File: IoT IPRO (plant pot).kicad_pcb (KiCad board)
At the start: 2 copper layers, 16 parts, among them J1 Barrel_Jack, Q1 Q_DUAL_NMOS_S1G1S2G2D1D1D2D2, U1 DS18S20, U3 AP9101C-SOT25

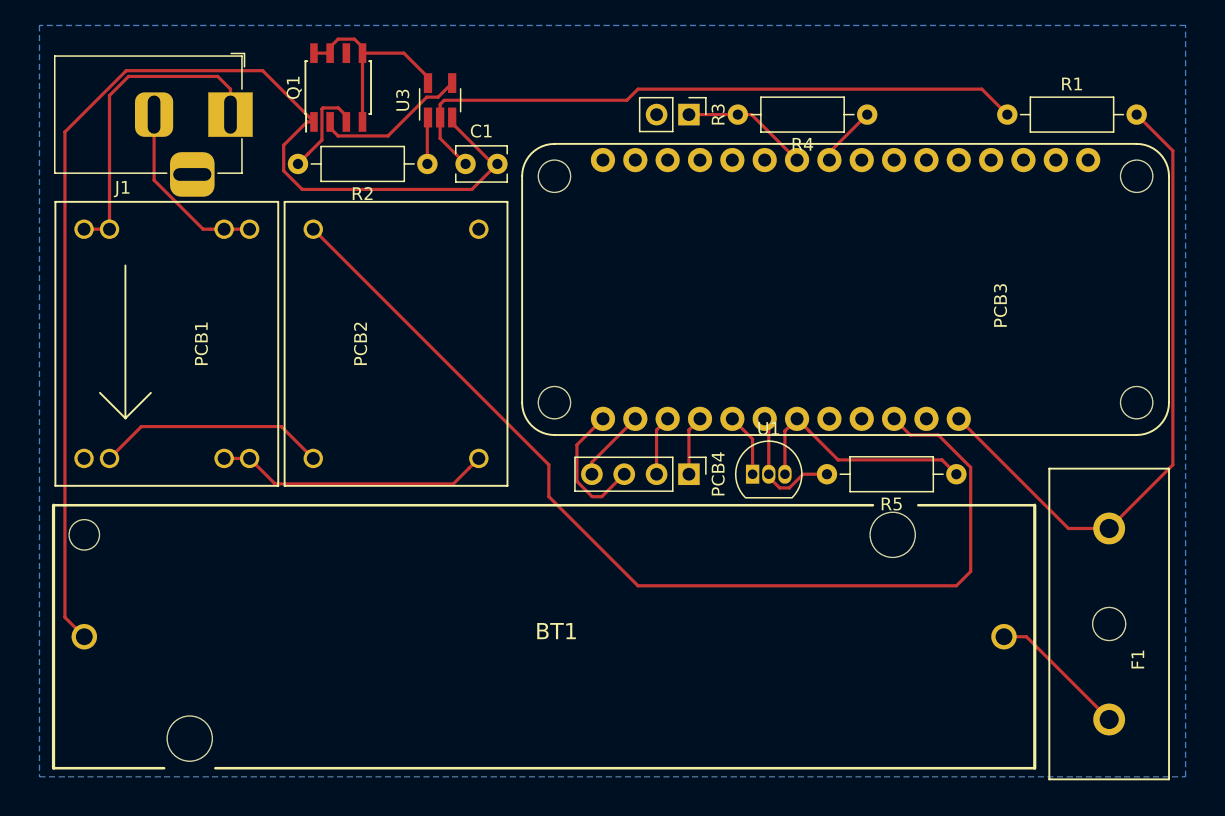
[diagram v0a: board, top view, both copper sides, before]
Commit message: Update PCB, PDFs
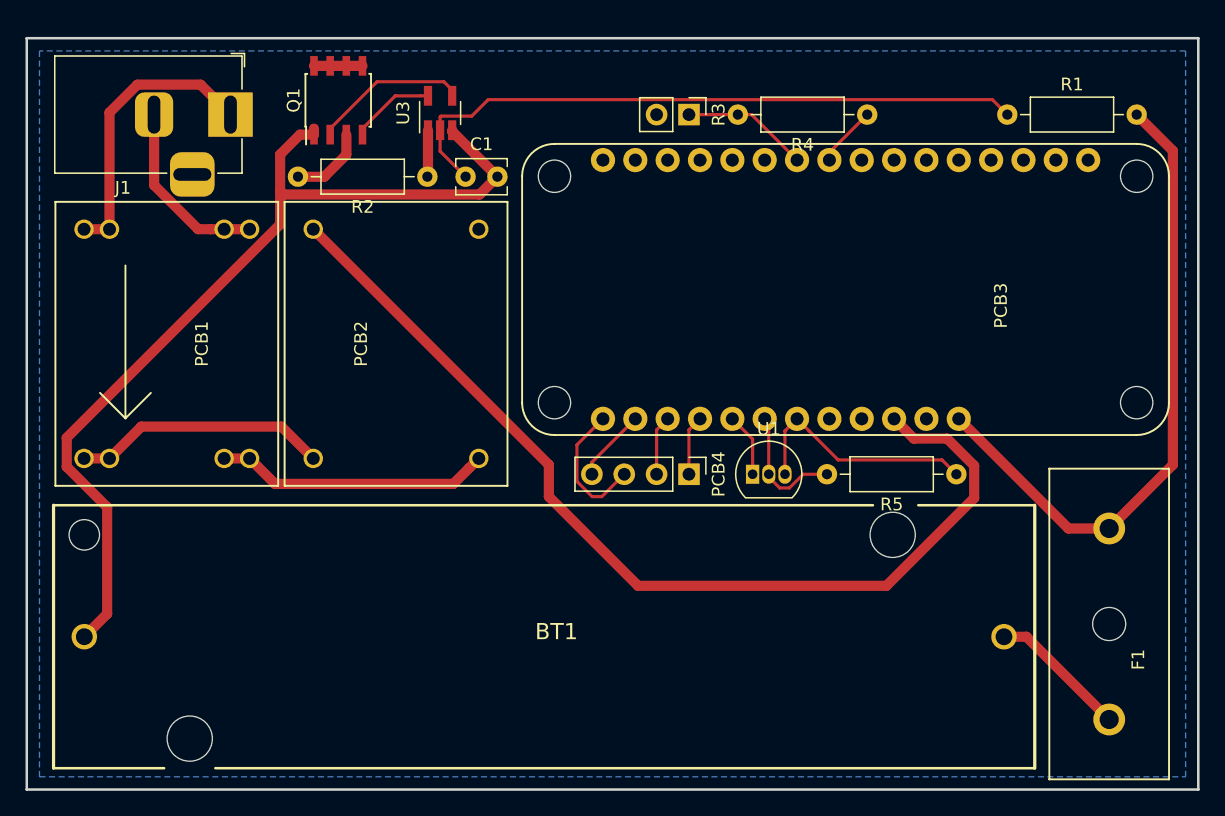
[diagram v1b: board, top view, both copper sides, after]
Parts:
- moved C1 1.00 mm to (92.5, 39.9)
- moved Q1 1.00 mm to (82.5, 33.9)
- moved R2 1.00 mm to (89.5, 39.9)
- moved U3 1.00 mm to (90.5, 34.9)
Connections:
- Q1 pad 5: Net-(Q1-Pad4) -> Net-(Q1-Pad5)
- Q1 pad 6: (no net) -> Net-(Q1-Pad5)
- Q1 pad 7: Net-(Q1-Pad4) -> Net-(Q1-Pad5)
- Q1 pad 8: Net-(Q1-Pad4) -> Net-(Q1-Pad5)
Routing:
- net Net-(BT1-Pad2): track 92.2 -> 73.5 mm
- net Net-(Q1-Pad4): track 17.1 -> 6.69 mm
- net Net-(Q1-Pad5): track 0.00 -> 3.81 mm
- net Net-(PCB2-Pad4): track 80.9 -> 78.2 mm
- net Net-(J1-Pad1): track 25.0 -> 22.5 mm
- net Net-(PCB1-Pad3): track 18.1 -> 20.1 mm
- net GND: track 7.78 -> 6.08 mm
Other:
- board outline added: 92 x 59 mm
